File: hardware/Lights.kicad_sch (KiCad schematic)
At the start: 0 parts

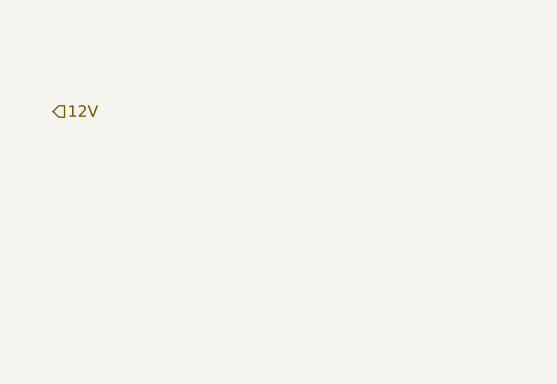
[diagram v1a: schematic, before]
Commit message: rawr
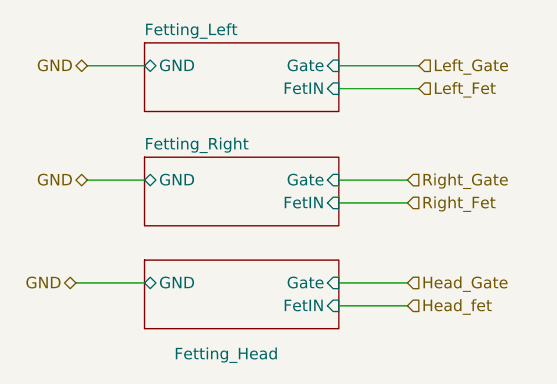
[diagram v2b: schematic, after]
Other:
- added sheet Fetting_Head (Fetting.kicad_sch)
- added sheet Fetting_Left (Fetting.kicad_sch)
- added sheet Fetting_Right (Fetting.kicad_sch)
